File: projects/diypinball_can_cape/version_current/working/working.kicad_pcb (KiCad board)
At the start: 2 copper layers, 86.4 x 54.6 mm, 42 parts, among them P1 BEAGLEBONE_BLACK, P2 PINBALL-CONNECTOR, P3 PINBALL-CONNECTOR, U1 MCP2562, U2 24C256, U3 AP3513E

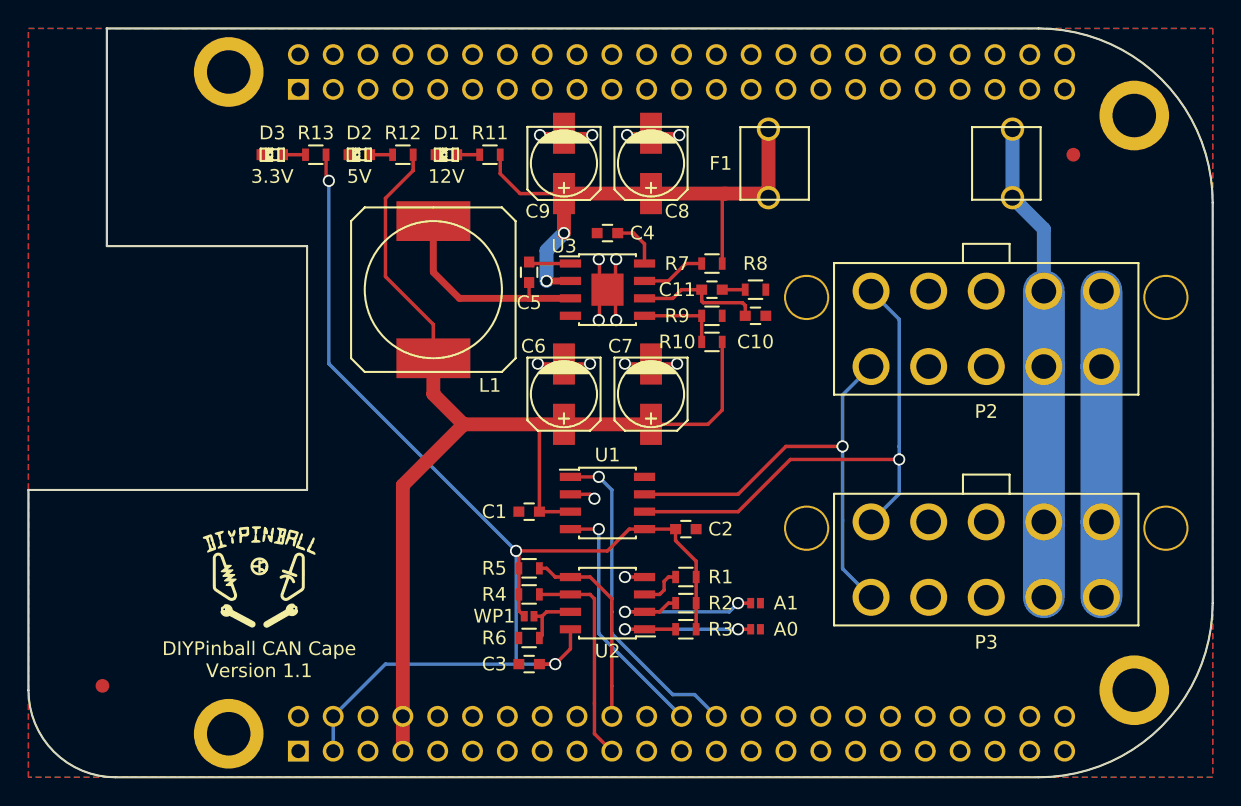
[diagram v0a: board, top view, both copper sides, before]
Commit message: updated all projects from src
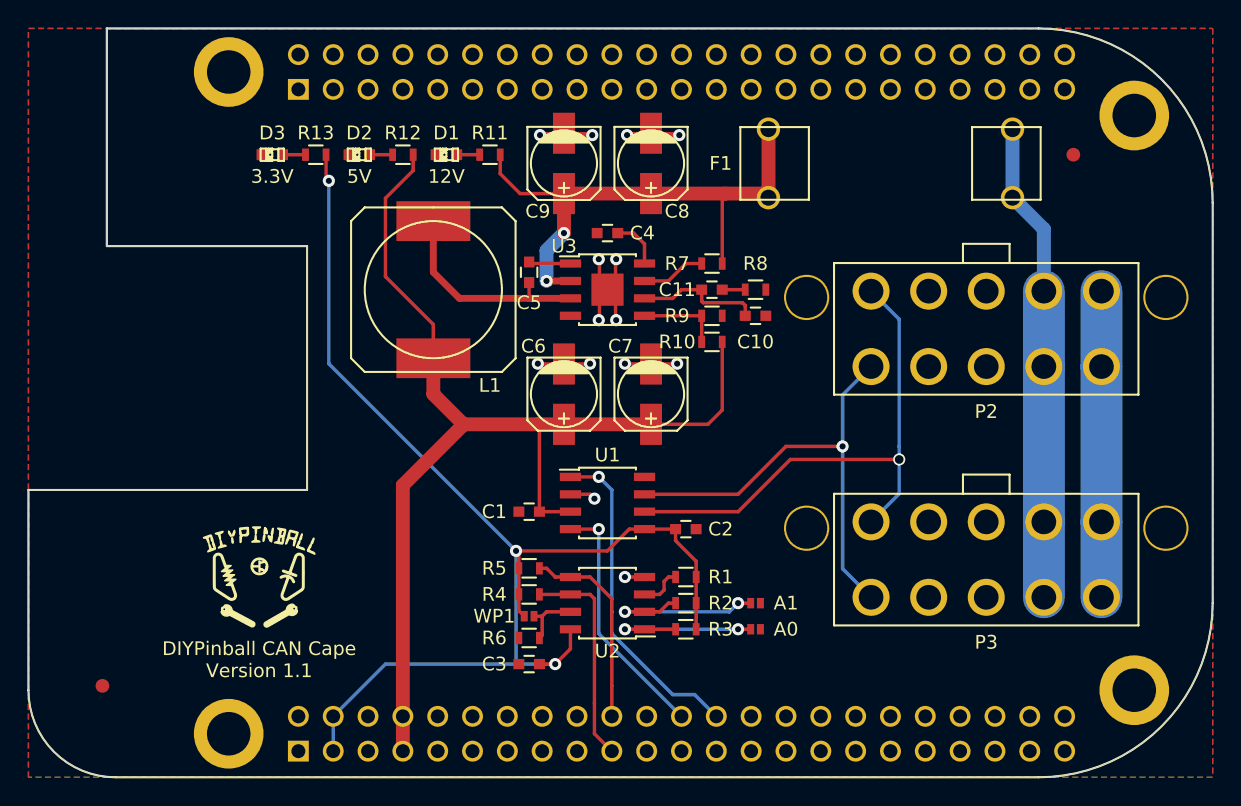
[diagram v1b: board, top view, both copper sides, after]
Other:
- net class Default added: clearance 0.254, trace_width 0.254, via_dia 0.889, via_drill 0.635
